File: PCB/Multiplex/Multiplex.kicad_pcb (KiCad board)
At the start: 2 copper layers, 48.3 x 40.6 mm, 20 parts, among them J1+1 Power, J1-1 Power, J2+1 I2C, J2-1 I2C, J3 Signal, J4 Track, K1 IM03, Q1 2N7002, U1 PIC16F1503-IP

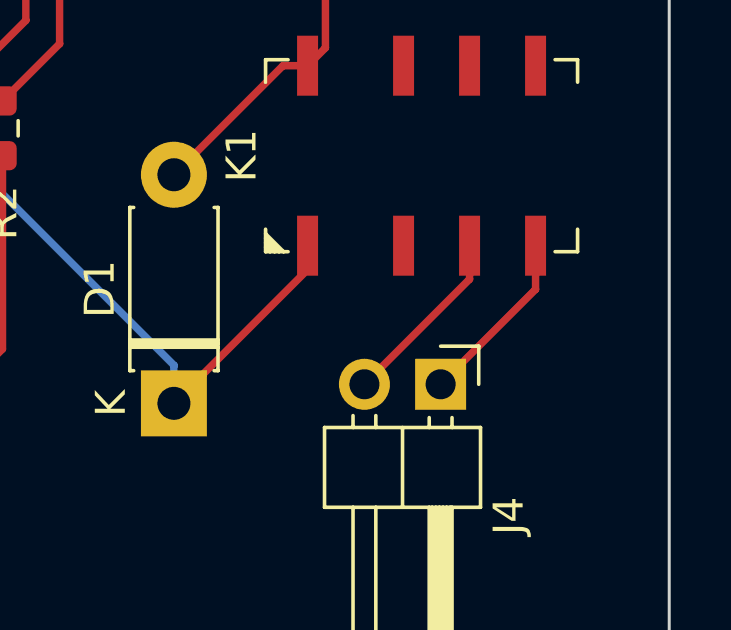
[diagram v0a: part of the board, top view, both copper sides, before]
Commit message: Added new PCB and updated older ones.
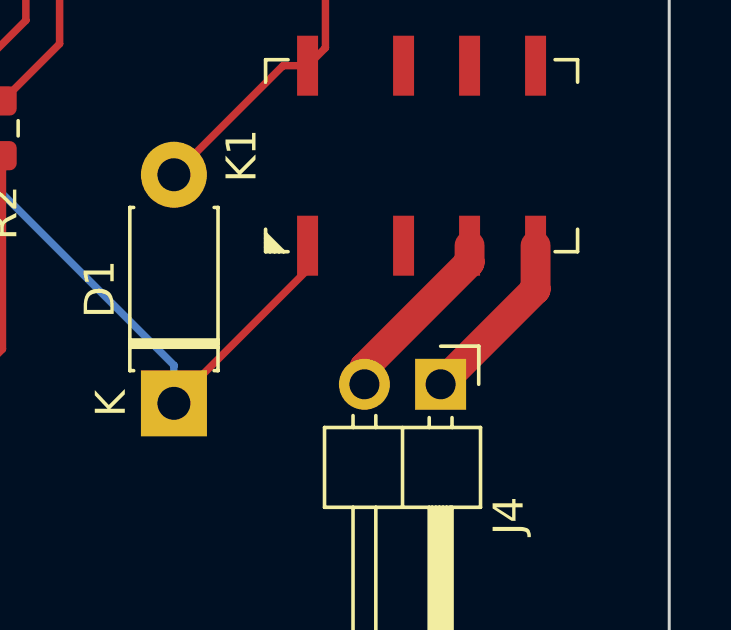
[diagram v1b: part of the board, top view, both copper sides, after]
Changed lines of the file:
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@@
 		)
 		(pad_to_mask_clearance 0.051)
-		(solder_mask_min_width 0.25)
 		(allow_soldermask_bridges_in_footprints no)
 		(pcbplotparams
@@
 	)
 	(segment
-		(start 180.965 117.485)
-		(end 177.8 120.65)
-		(width 0.25)
+		(start 177.8 120.65)
+		(end 180.965 117.485)
+		(width 1)
 		(layer "F.Cu")
 		(net 10)
 	)
 	(segment
-		(start 180.965 116.03)
-		(end 180.965 117.485)
-		(width 0.25)
+		(start 180.965 117.485)
+		(end 180.965 116.03)
+		(width 1)
 		(layer "F.Cu")
 		(net 10)
 	)
 	(segment
-		(start 178.765 117.145)
-		(end 175.26 120.65)
-		(width 0.25)
+		(start 175.26 120.65)
+		(end 175.26 120.09)
+		(width 1)
 		(layer "F.Cu")
 		(net 11)
 	)
 	(segment
-		(start 178.765 116.03)
-		(end 178.765 117.145)
-		(width 0.25)
+		(start 175.26 120.09)
+		(end 178.765 116.585)
+		(width 1)
+		(layer "F.Cu")
+		(net 11)
+	)
+	(segment
+		(start 178.765 116.585)
+		(end 178.765 116.03)
+		(width 1)
 		(layer "F.Cu")
 		(net 11)
